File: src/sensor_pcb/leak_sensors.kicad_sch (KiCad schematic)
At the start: 6 parts, among them Q1 NPN BJT 40V 200mA

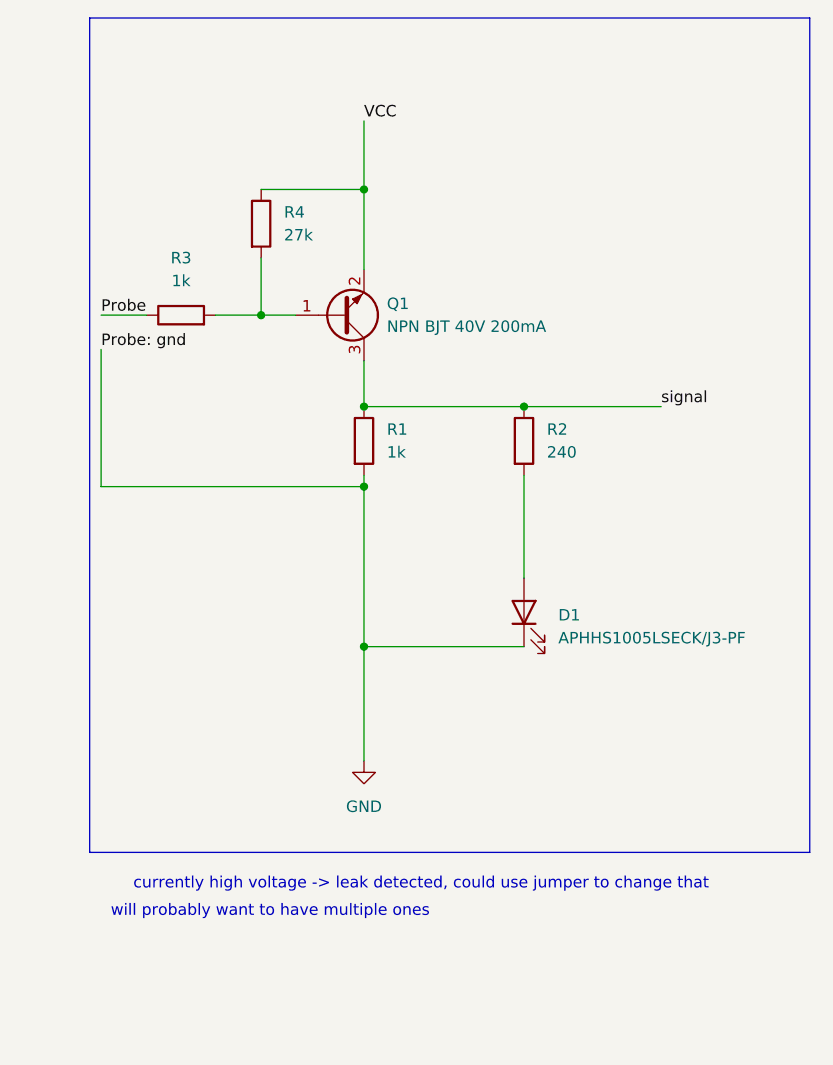
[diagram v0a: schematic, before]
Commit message: 8 pin connectors added
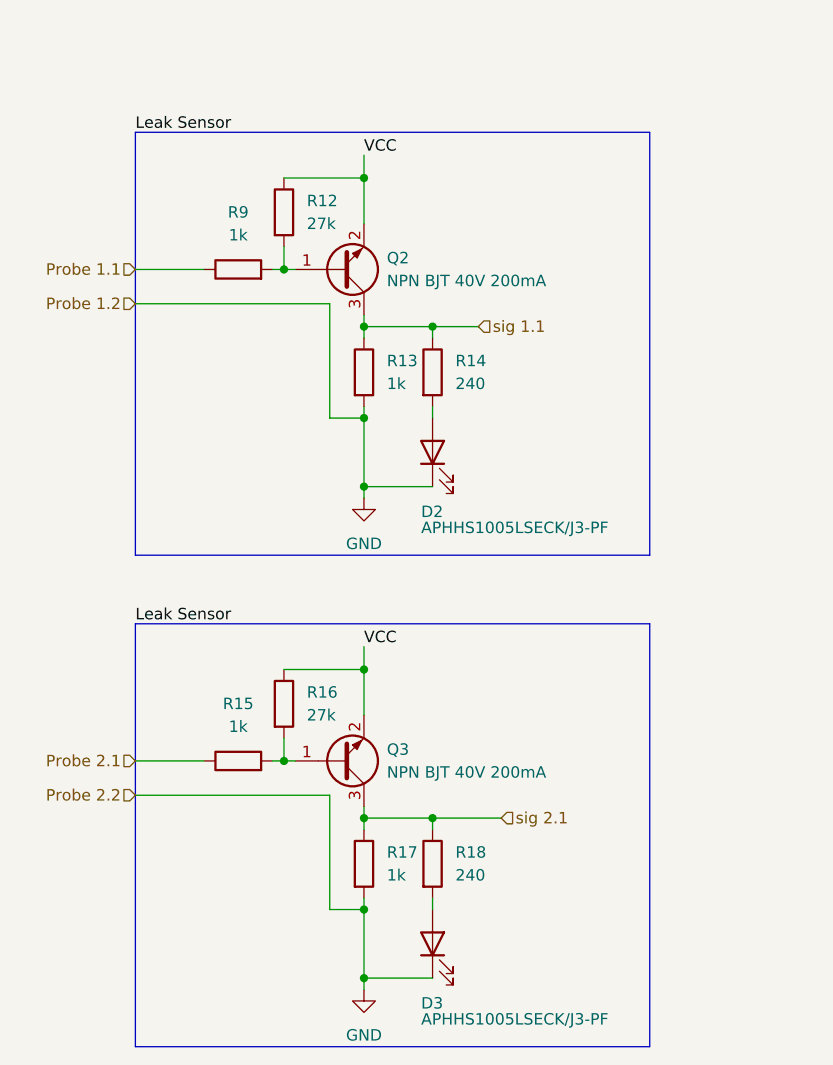
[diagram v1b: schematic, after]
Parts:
- removed D1: APHHS1005LSECK/J3-PF, LED_SMD:LED_0402_1005Metric, symbol #dzdb:s_dio/D-KIN-APHHS1005LSECK/J3-PF
- removed Q1: NPN BJT 40V 200mA, Package_TO_SOT_SMD:SOT-23, symbol #dzdb:s_misc/Q-NPN-200-SOT23
- removed R1, R3: 1k, Resistor_SMD:R_0603_1608Metric, symbol #dzdb:g_res/R-1k-0603
- removed R2: 240, Resistor_SMD:R_0603_1608Metric, symbol #dzdb:g_res/R-240-0603
- removed R4: 27k, Resistor_SMD:R_0603_1608Metric, symbol #dzdb:g_res/R-27k-0603
- added D2, D3: APHHS1005LSECK/J3-PF, LED_SMD:LED_0402_1005Metric, symbol #dzdb:s_dio/D-KIN-APHHS1005LSECK/J3-PF
- added Q2, Q3: NPN BJT 40V 200mA, Package_TO_SOT_SMD:SOT-23, symbol #dzdb:s_misc/Q-NPN-200-SOT23
- added R12, R16: 27k, Resistor_SMD:R_0603_1608Metric, symbol #dzdb:g_res/R-27k-0603
- added R13, R15, R17, R9: 1k, Resistor_SMD:R_0603_1608Metric, symbol #dzdb:g_res/R-1k-0603
- added R14, R18: 240, Resistor_SMD:R_0603_1608Metric, symbol #dzdb:g_res/R-240-0603
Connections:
- net GND: now also D2.1 (K), D3.1 (K), R13.2, R17.2
- net VCC: now also Q2.2 (E), Q3.2 (E), R12.1, R16.1
- new net: Q3.1 (B), R15.2, R16.2
- new net: D2.2 (A), R14.2
- new net: Q2.1 (B), R12.2, R9.2
- new net: D3.2 (A), R18.2
- new net Probe 1.1: R9.1
- new net Probe 2.1: R15.1
- new net sig 1.1: Q2.3 (C), R13.1, R14.1
- new net sig 2.1: Q3.3 (C), R17.1, R18.1
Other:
- note removed: "currently high voltage -> leak detected, could use jumper to change that"
- note removed: "will probably want to have multiple ones"
